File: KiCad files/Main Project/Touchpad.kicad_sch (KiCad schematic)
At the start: 5 parts, among them U17 PCF8575

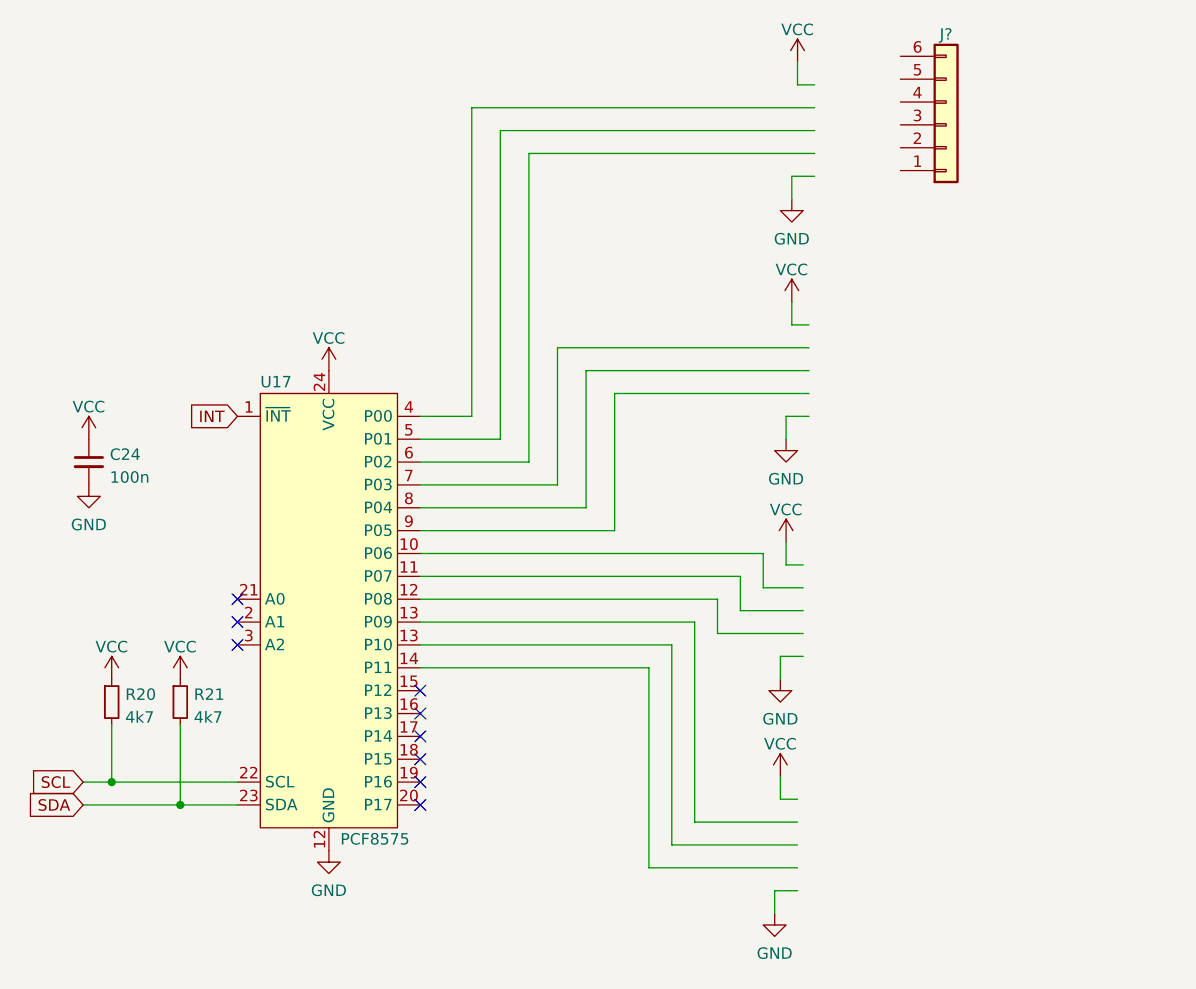
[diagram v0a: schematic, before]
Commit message: update
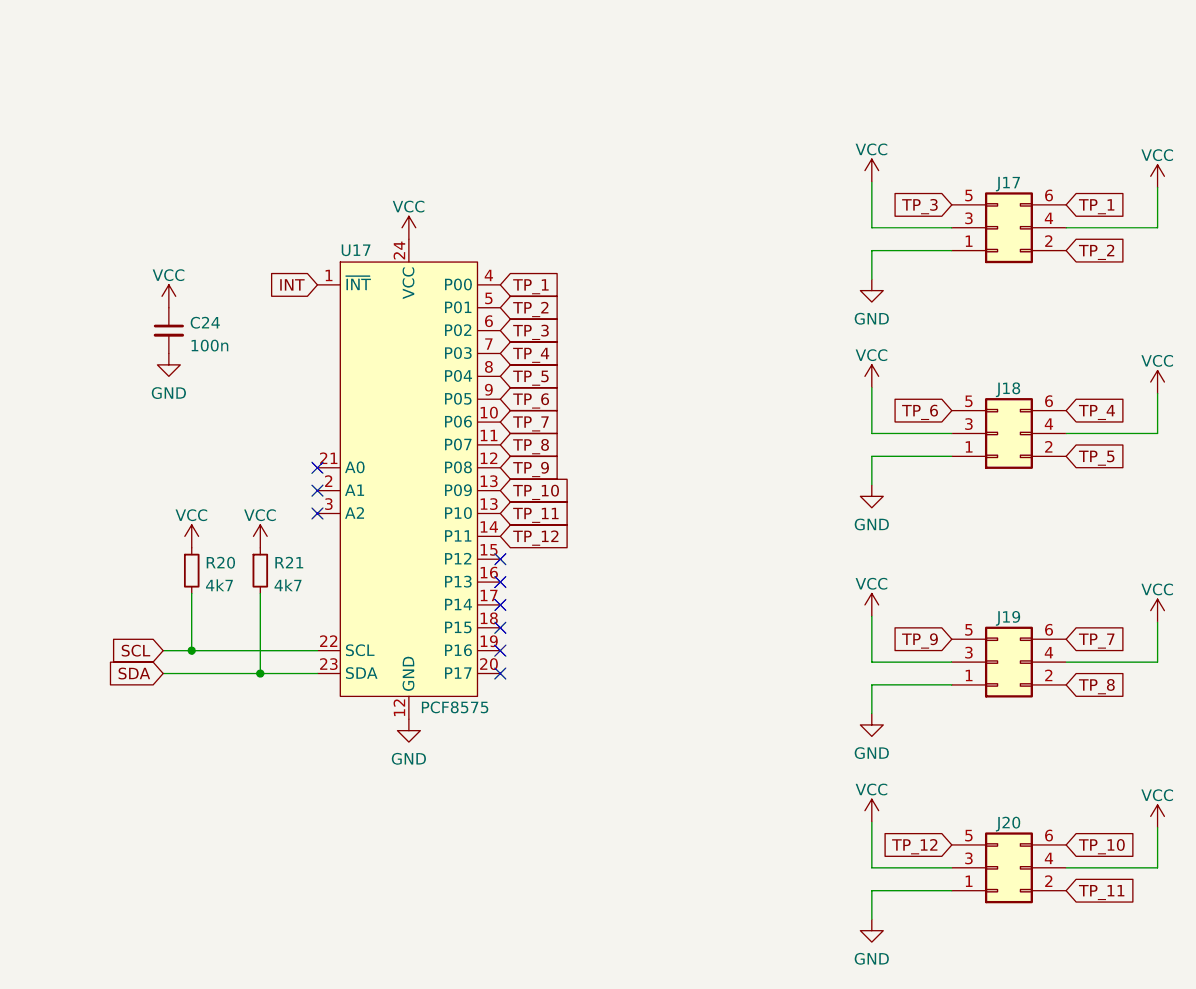
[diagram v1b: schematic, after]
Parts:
- removed J?: Conn_01x06, symbol Connector_Generic:Conn_01x06
- added J17, J18, J19, J20: Conn_02x03_Odd_Even, Connector_PinSocket_1.27mm:PinSocket_2x03_P1.27mm_Vertical, symbol Connector_Generic:Conn_02x03_Odd_Even
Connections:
- net GND: now also J17.1 (Pin_1), J18.1 (Pin_1), J19.1 (Pin_1), J20.1 (Pin_1)
- net VCC: now also J17.3 (Pin_3), J17.4 (Pin_4), J18.3 (Pin_3), J18.4 (Pin_4), J19.3 (Pin_3), J19.4 (Pin_4), J20.3 (Pin_3), J20.4 (Pin_4)
- net TP_7: now reaches U17.10 (P06)
- net TP_7: now also J19.6 (Pin_6)
- net TP_8: now reaches U17.11 (P07)
- net TP_8: now also J19.2 (Pin_2)
- net TP_9: now reaches U17.12 (P08)
- net TP_9: now also J19.5 (Pin_5)
- net TP_11: now reaches U17.13 (P10)
- net TP_11: now also J20.2 (Pin_2)
- net TP_12: now reaches U17.14 (P11)
- net TP_12: now also J20.5 (Pin_5)
- net TP_1: now reaches U17.4 (P00)
- net TP_1: now also J17.6 (Pin_6)
- net TP_2: now reaches U17.5 (P01)
- net TP_2: now also J17.2 (Pin_2)
- net TP_3: now reaches U17.6 (P02)
- net TP_3: now also J17.5 (Pin_5)
- net TP_4: now reaches U17.7 (P03)
- net TP_4: now also J18.6 (Pin_6)
- net TP_5: now reaches U17.8 (P04)
- net TP_5: now also J18.2 (Pin_2)
- net TP_6: now reaches U17.9 (P05)
- net TP_6: now also J18.5 (Pin_5)
- new net TP_10: J20.6 (Pin_6), U17.13 (P10)
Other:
- moved on the sheet: C24, R20, R21, U17
